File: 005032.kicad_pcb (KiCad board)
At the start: 2 copper layers, 43 x 26 mm, 47 parts, among them J1 alim+conn, J2 PROG_ESP02, J4 JTAG, SW1 DMR02, SW2 434153017835, SW3 434153017835, U1 ESP32-WROOM-32E, U2 AP63201, U3 AP63357

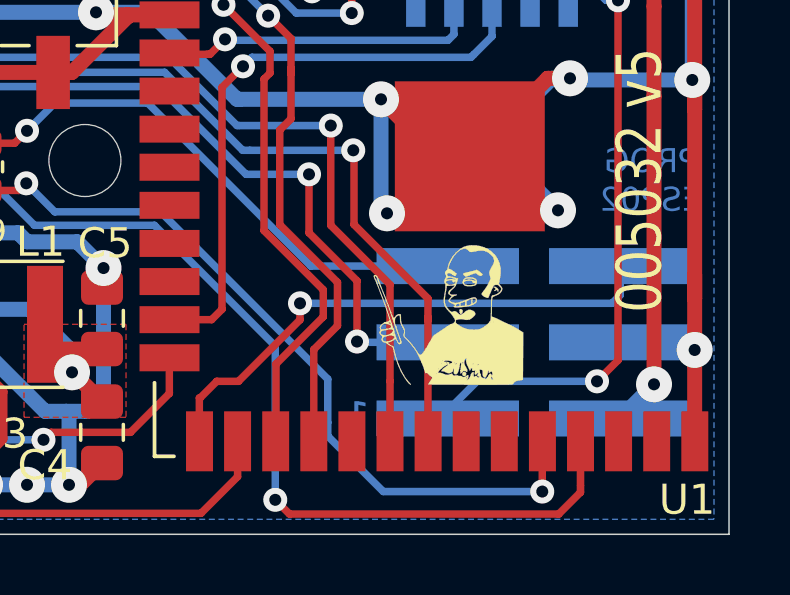
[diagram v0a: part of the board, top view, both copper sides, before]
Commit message: v5 - commit prima di esecuzione modifiche v6
Signed-off-by: Andrea Toninelli <tonazza@yahoo.it>
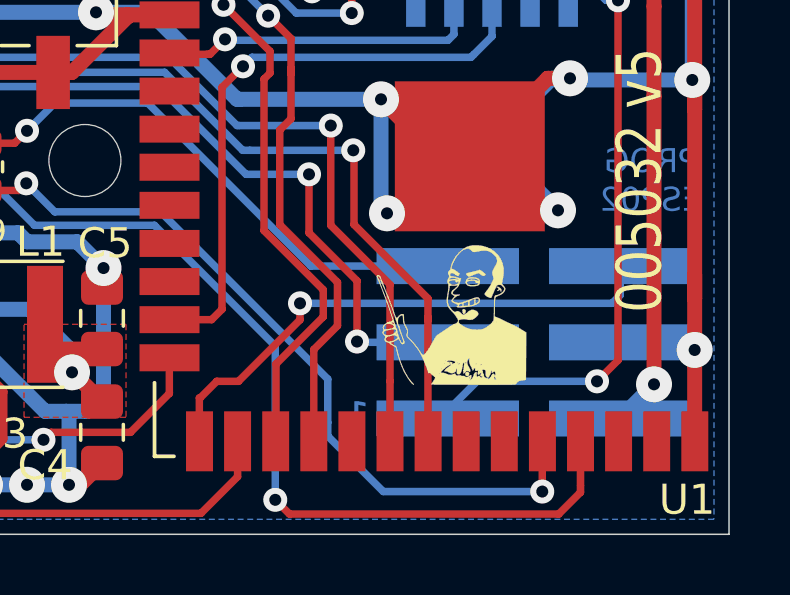
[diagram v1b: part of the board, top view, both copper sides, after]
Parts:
- moved G*** 0.10 mm to (133.7, 92.5)
